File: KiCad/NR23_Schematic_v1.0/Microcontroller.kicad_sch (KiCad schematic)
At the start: 4 parts

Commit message: added benchtop model schematic
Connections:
- new net: U?. (GND), U?. (To_TI_CAN_L) (x2)
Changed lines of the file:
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@@
   (paper "A")
   (title_block
-    (date "2023-02-28")
+    (date "2023-03-03")
   )
   (wire (pts (xy 137.16 140.97) (xy 137.16 125.73))

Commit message: Battery update
Made big changes to the battery. Added all 16 battery pins. Started connecting the battery
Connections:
- new net: U?. (GND), U?. (To_TI_CAN_L) (x2)

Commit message: added more to the safety circuit
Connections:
- new net: U?. (GND), U?. (To_TI_CAN_L) (x2)

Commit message: Added Dash to Schematic
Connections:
- new net: U?. (GND), U?. (To_TI_CAN_L) (x2)

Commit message: worked some more on emergency stop switches
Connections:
- new net: U?. (GND), U?. (To_TI_CAN_L) (x2)

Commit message: added TI board box on the Tractive System Schematc
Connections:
- new net: U?. (GND), U?. (To_TI_CAN_L) (x2)

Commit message: endish of day 05APR23
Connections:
- new net: U?. (GND), U?. (To_TI_CAN_L) (x2)

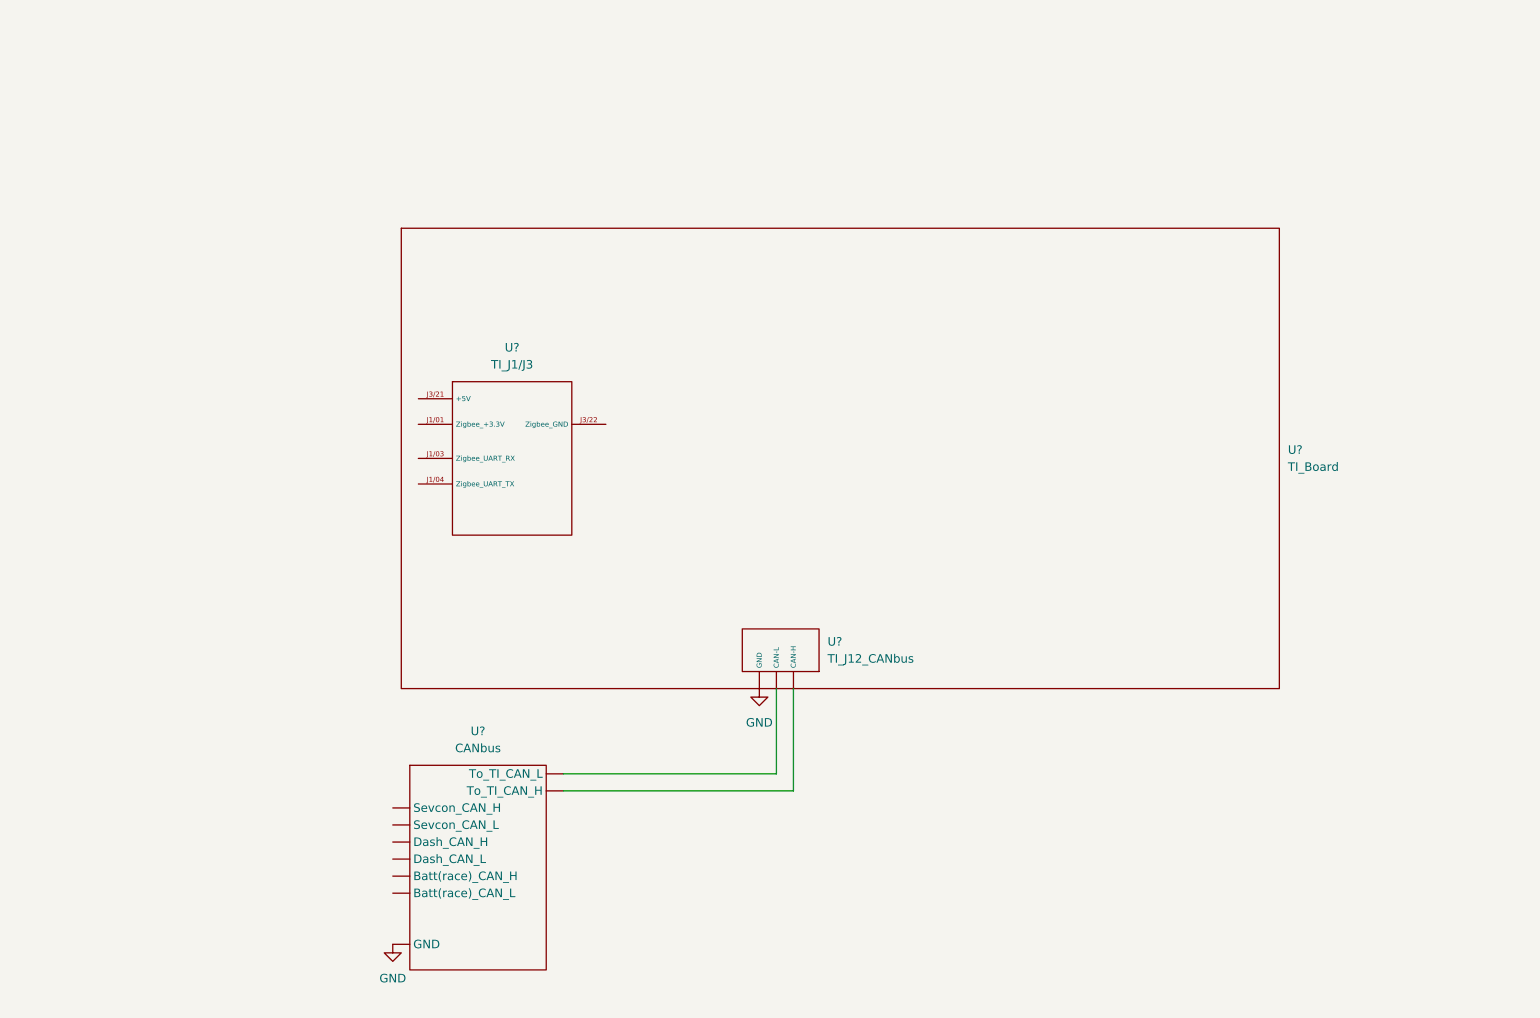
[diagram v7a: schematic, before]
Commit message: end of day 05APR23
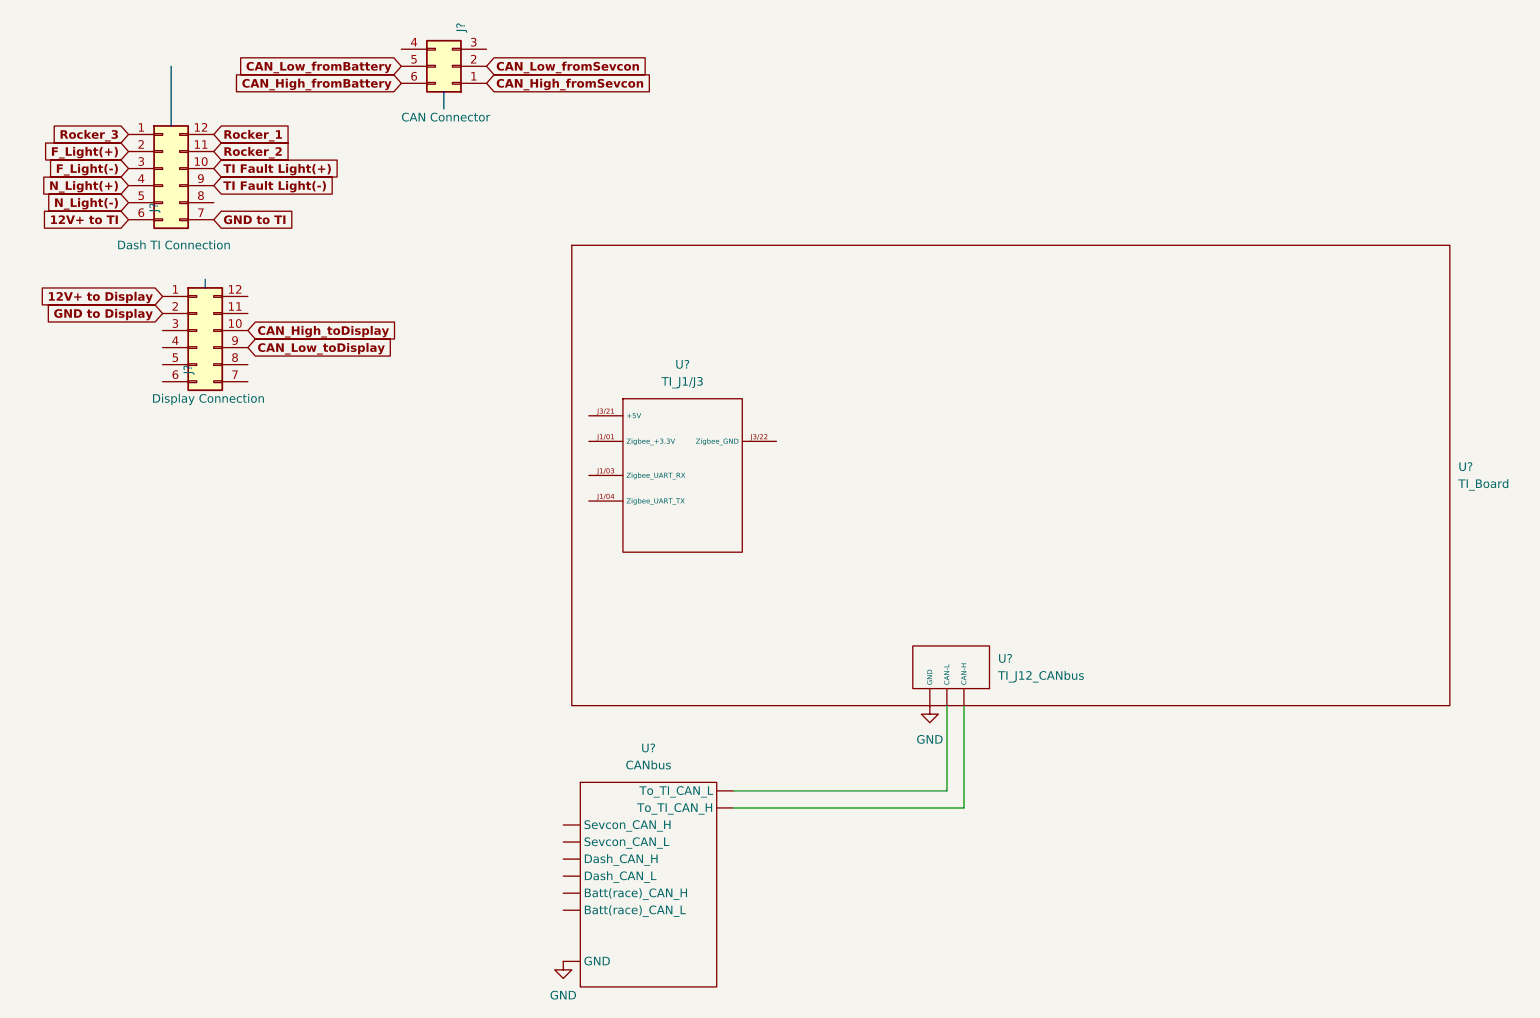
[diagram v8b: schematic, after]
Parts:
- added J?: Display Connection, symbol Connector_Generic:Conn_02x06_Counter_Clockwise
- added J?: Dash TI Connection, symbol Connector_Generic:Conn_02x06_Counter_Clockwise
- added J?: CAN Connector, symbol Connector_Generic:Conn_02x03_Counter_Clockwise
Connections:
- new net: U?. (GND), U?. (To_TI_CAN_L) (x2)
- new net 12V+ to Display: J?.1 (Pin_1)
- new net 12V+ to TI: J?.6 (Pin_6)
- new net CAN_High_fromBattery: J?.6 (Pin_6)
- new net CAN_High_fromSevcon: J?.1 (Pin_1)
- new net CAN_High_toDisplay: J?.10 (Pin_10)
- new net CAN_Low_fromBattery: J?.5 (Pin_5)
- new net CAN_Low_fromSevcon: J?.2 (Pin_2)
- new net CAN_Low_toDisplay: J?.9 (Pin_9)
- new net F_Light(+): J?.2 (Pin_2)
- new net F_Light(-): J?.3 (Pin_3)
- new net GND to Display: J?.2 (Pin_2)
- new net GND to TI: J?.7 (Pin_7)
- new net N_Light(+): J?.4 (Pin_4)
- new net N_Light(-): J?.5 (Pin_5)
- new net Rocker_1: J?.12 (Pin_12)
- new net Rocker_2: J?.11 (Pin_11)
- new net Rocker_3: J?.1 (Pin_1)
- new net TI Fault Light(+): J?.10 (Pin_10)
- new net TI Fault Light(-): J?.9 (Pin_9)
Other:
- moved on the sheet: U?
